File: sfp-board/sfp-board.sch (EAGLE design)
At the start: 6 parts

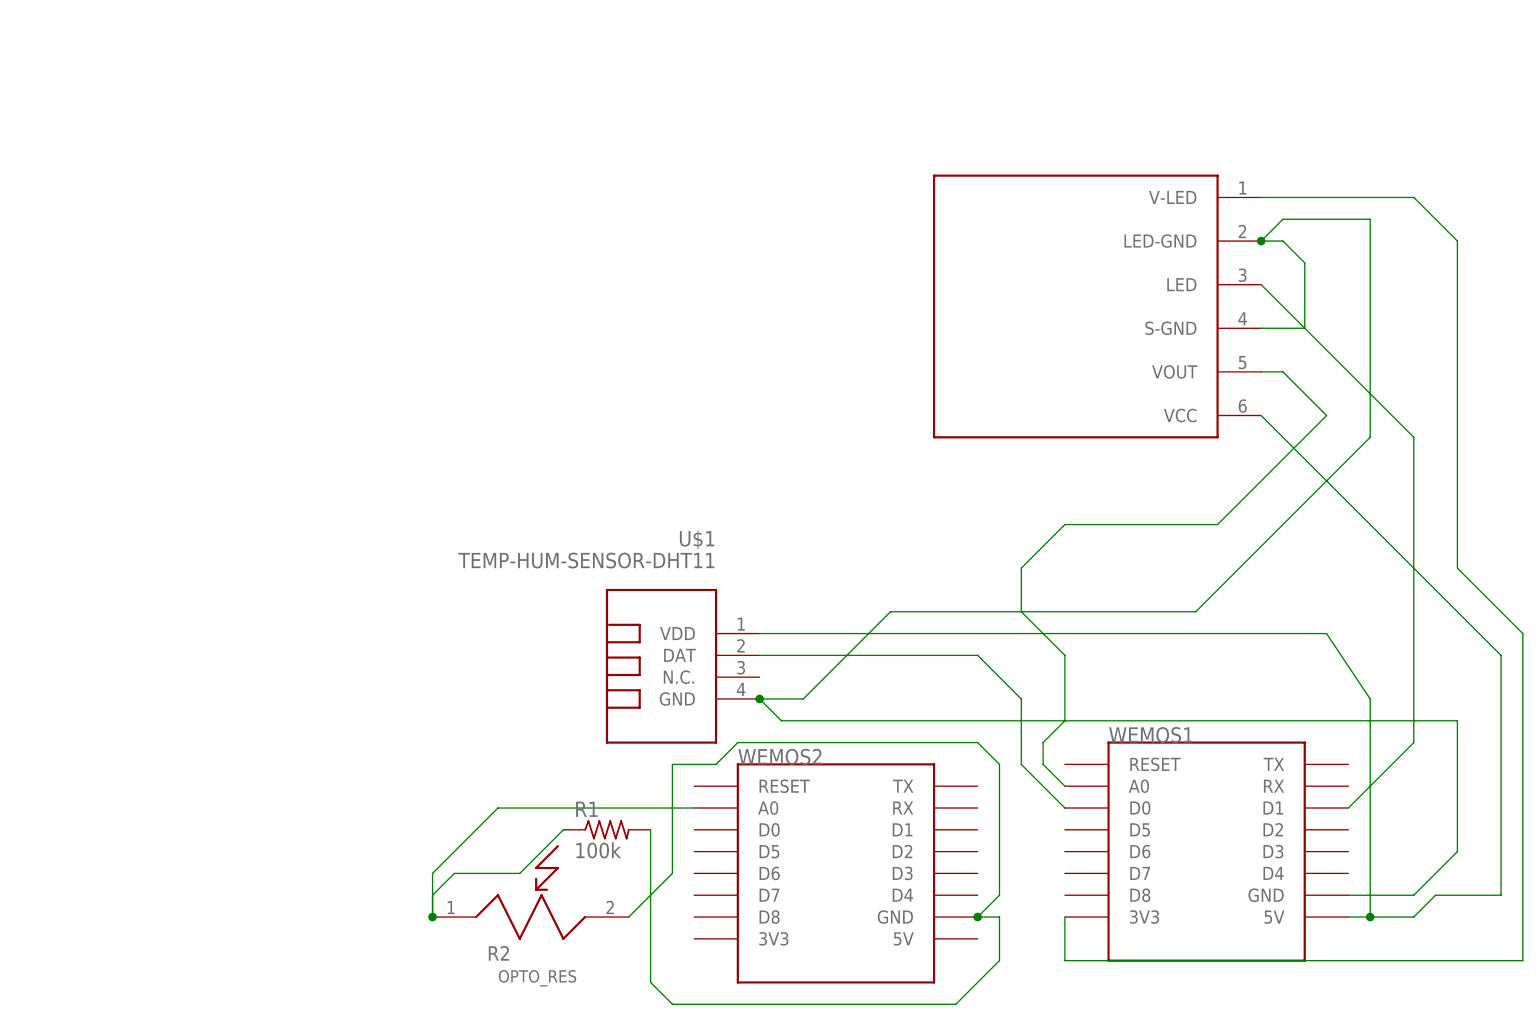
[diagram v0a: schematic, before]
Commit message: Initial version sfp board
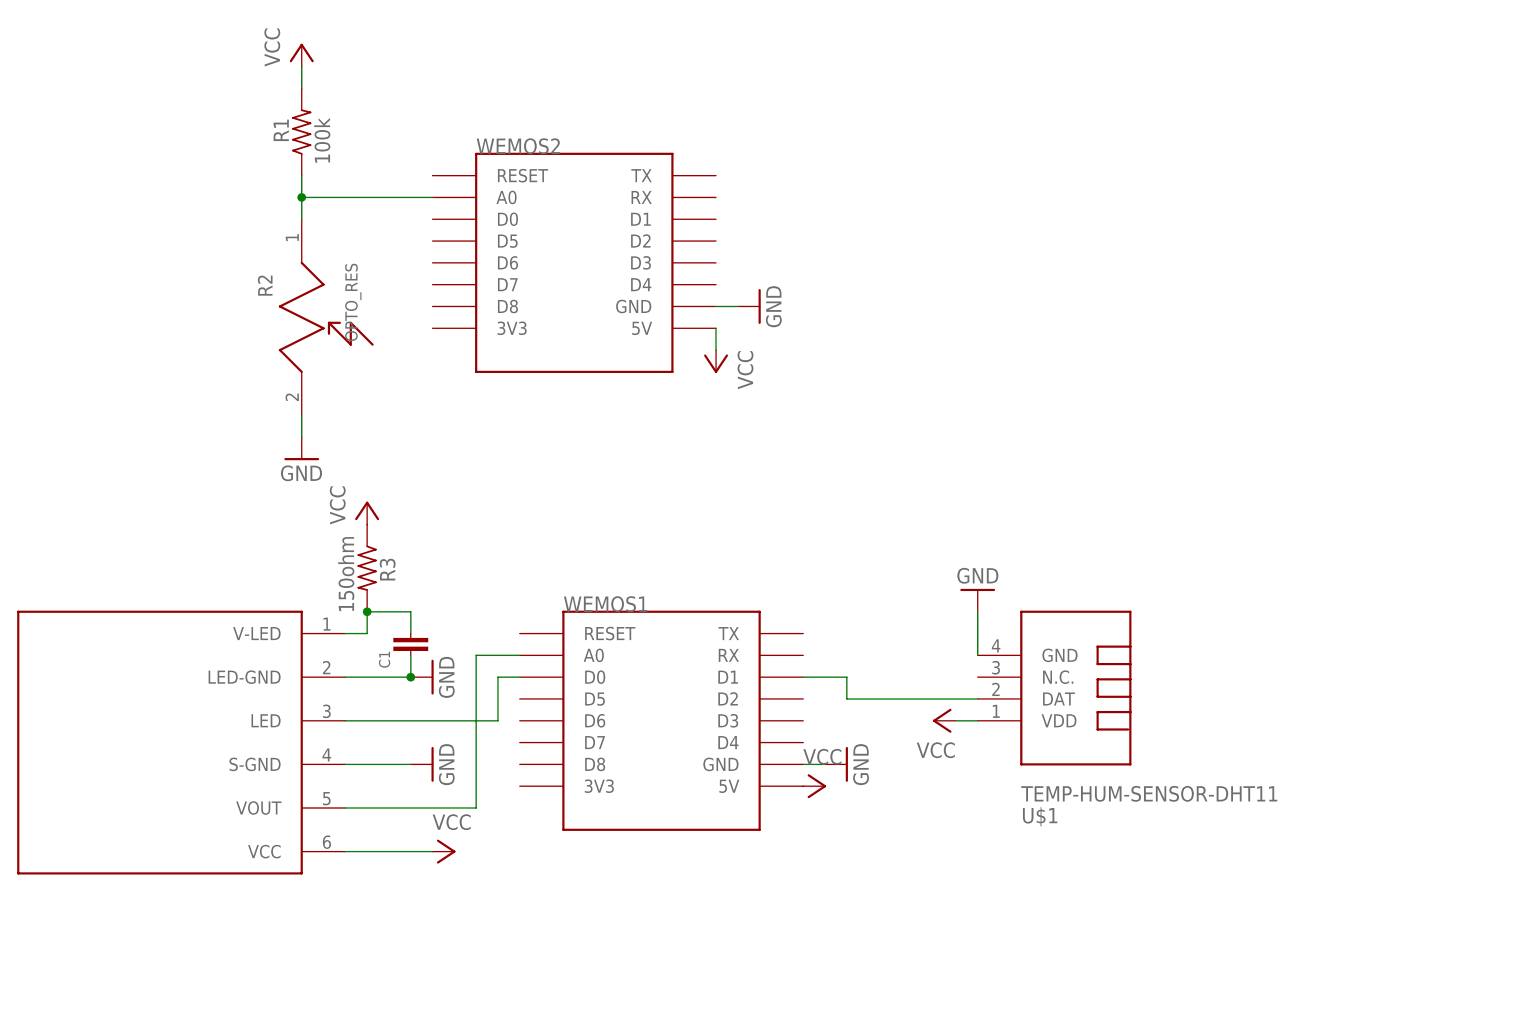
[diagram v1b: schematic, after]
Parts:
- added C1: (no value), digital-toy:CAPPTH1
- added R3: 150ohm, rcl:R-US_0411/15
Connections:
- removed net N$1 (its old number): U$1.GND, U$2.LED-GND, U$2.S-GND, WEMOS1.GND
- removed net N$2 (its old number): R1.2, R2.P2, WEMOS2.GND
- removed net N$6: U$1.VDD, U$2.VCC, WEMOS1.5V
- new net GND: C1.2, R2.P2, U$1.GND, U$2.LED-GND, U$2.S-GND, WEMOS1.GND, WEMOS2.GND
- new net VCC: R1.2, R3.1, U$1.VDD, U$2.VCC, WEMOS1.5V, WEMOS2.5V
- net N$3: now also U$2.LED; no longer U$1.DAT
- net N$4: now also C1.1, R3.2; no longer WEMOS1.3V3
- net N$7: now also U$1.DAT; no longer U$2.LED
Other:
- moved on the sheet: R1, R2, U$1, WEMOS1, WEMOS2
